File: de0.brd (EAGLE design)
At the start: 148.8 x 90.3 mm, 137 parts, among them IC1 PL2303SA__LF, J1 JUMPER_IN_50, J2 UX60SC-MB-5ST, J3 REG_OUT_33, U1 P0082, U2 RFM95W-915S2, U3 TPS76201DBVR, U4 TPS76201DBVR, U5 TPS76201DBVR

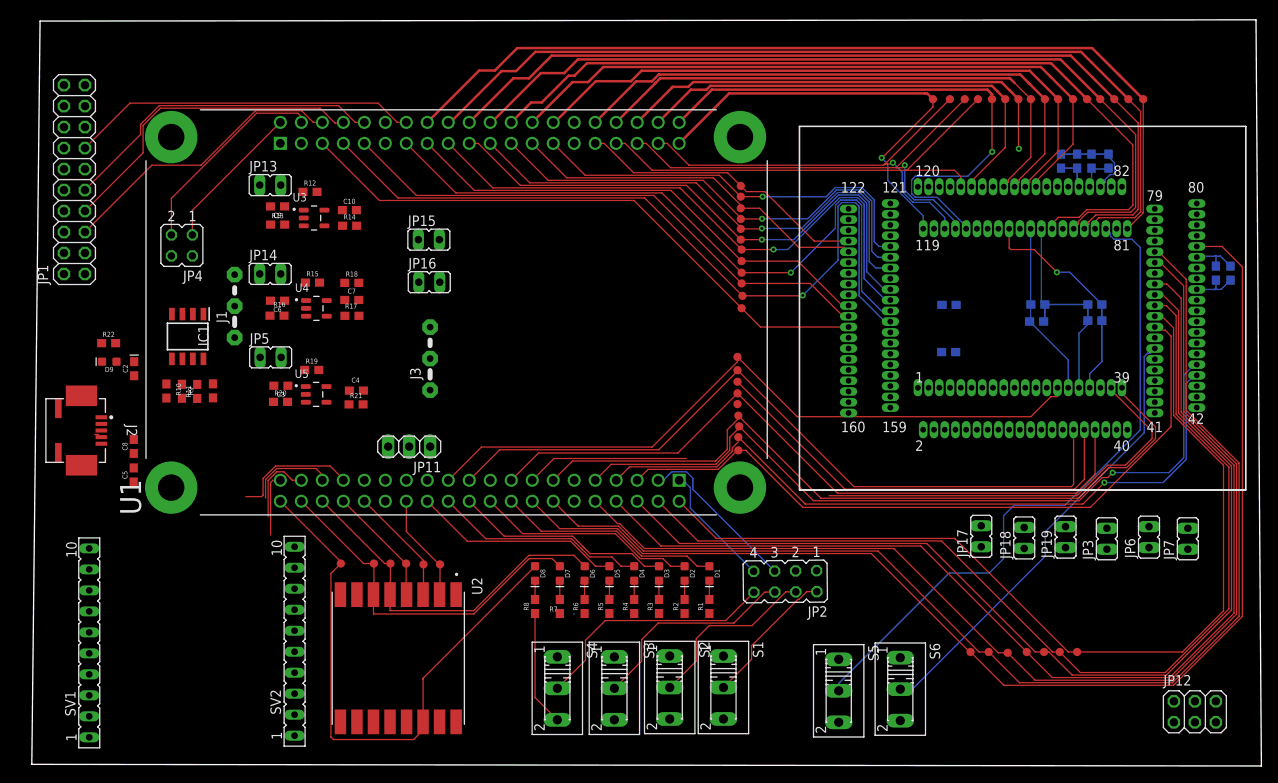
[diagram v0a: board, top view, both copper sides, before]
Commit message: Update layout
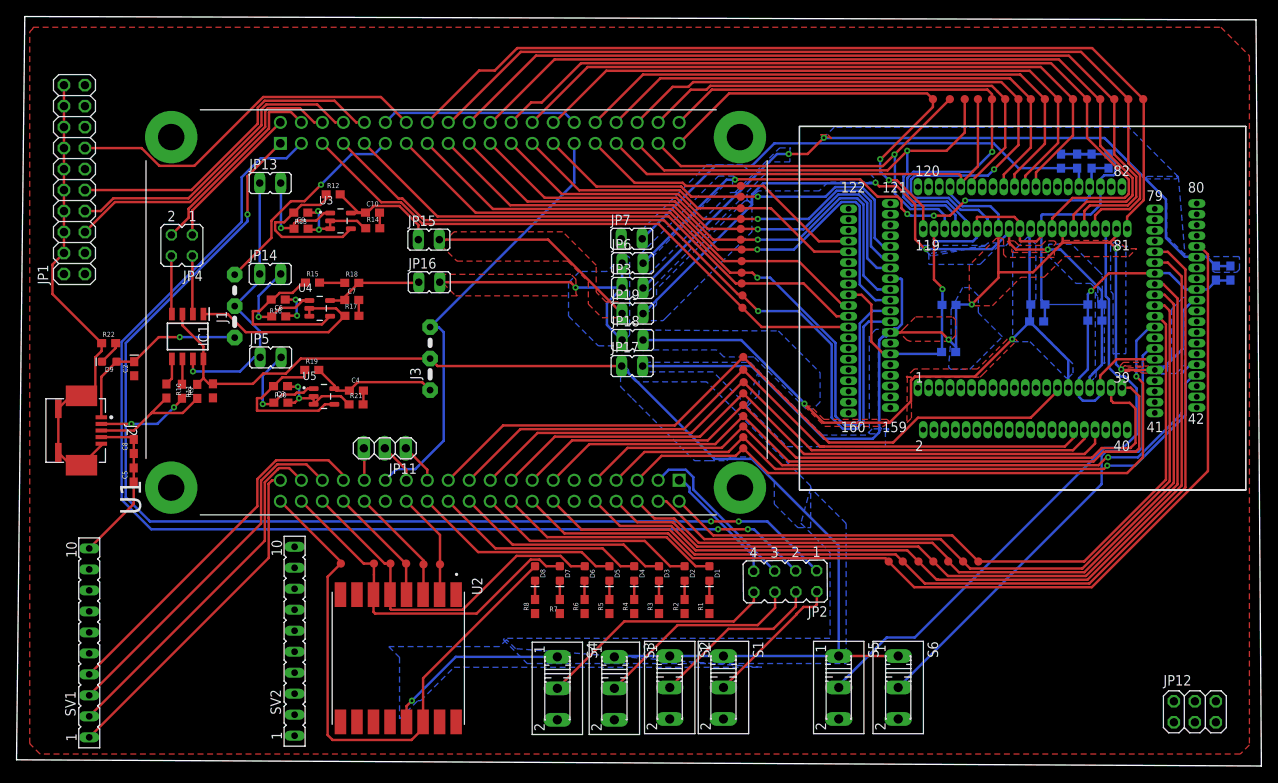
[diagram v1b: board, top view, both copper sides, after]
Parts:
- moved JP7 76.5 mm to (5.80, 28.7), turned to 270 degrees
- moved JP6 70.7 mm to (5.90, 25.8), turned to 270 degrees
- moved JP3 64.9 mm to (5.90, 22.8), turned to 270 degrees
- moved JP19 59.0 mm to (5.90, 19.6), turned to 270 degrees
- moved JP18 53.1 mm to (5.90, 16.4), turned to 270 degrees
- moved JP17 47.0 mm to (5.85, 13.3), turned to 270 degrees
- moved U$10 16.2 mm to (47.8, -10.3)
- moved U$11 16.0 mm to (45.9, -10.3)
- moved U$12 16.0 mm to (44.1, -10.3)
- moved U$13 15.7 mm to (42.3, -10.3)
- moved U$14 15.5 mm to (40.5, -10.3)
- moved U$15 15.1 mm to (38.6, -10.3)
- moved U$16 14.8 mm to (36.9, -10.3)
- moved C9 3.93 mm to (-34.2, 29.9), turned to 0 degrees
- moved U3 3.22 mm to (-29.4, 30.9)
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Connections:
- net GND: now also U$1.35, U$1.67
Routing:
- net GND: track 59.5 -> 296.2 mm, vias 0 -> 8
- net VO_33: track 0.00 -> 168.1 mm, vias 0 -> 1
- net VCCQ: track 0.00 -> 140.5 mm, vias 0 -> 4
- net N$10: track 0.00 -> 139.1 mm, vias 0 -> 2
- net N$9: track 0.00 -> 137.9 mm, vias 0 -> 3
- net VDD: track 5.82 -> 87.9 mm, vias 0 -> 2
- net VBP: track 4.43 -> 67.2 mm, vias 0 -> 4
- net VDDH: track 21.2 -> 80.9 mm, vias 0 -> 2
- net VDDLS: track 27.1 -> 86.6 mm, vias 1 -> 3
- net VBN: track 4.29 -> 61.0 mm
- net VO_FPGA_33: track 0.00 -> 53.5 mm
- net VDD5: track 0.00 -> 34.0 mm, vias 0 -> 1
- net SPI_SCK: track 7.63 -> 41.3 mm
- net SPI_MOSI: track 9.23 -> 42.9 mm
- net VO_12: track 0.00 -> 33.2 mm, vias 0 -> 1
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- added copper zone on layer 1, net GND
- added copper zone on layer 16, net V0_12
- added copper zone on layer 16, net VBN
- added copper zone on layer 16, net VBP
- added copper zone on layer 1, net VCCQ
- added copper zone on layer 16, net VCCQ
- added copper zone on layer 1, net VDD
- added copper zone on layer 16, net VDD
- added copper zone on layer 1, net VDDH
- added copper zone on layer 16, net VDDH
- added copper zone on layer 1, net VDDLS
- added copper zone on layer 16, net VDDLS
- added copper zone on layer 1, net VO_07
- added copper zone on layer 1, net VO_12
- added copper zone on layer 16, net VO_33
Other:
- board size 148.8 x 90.3 mm -> 150.7 x 90.7 mm
